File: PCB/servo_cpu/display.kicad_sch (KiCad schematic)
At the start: 15 parts, among them SW1 ENTER, SW2 ESC, SW3 UP, SW4 DOWN

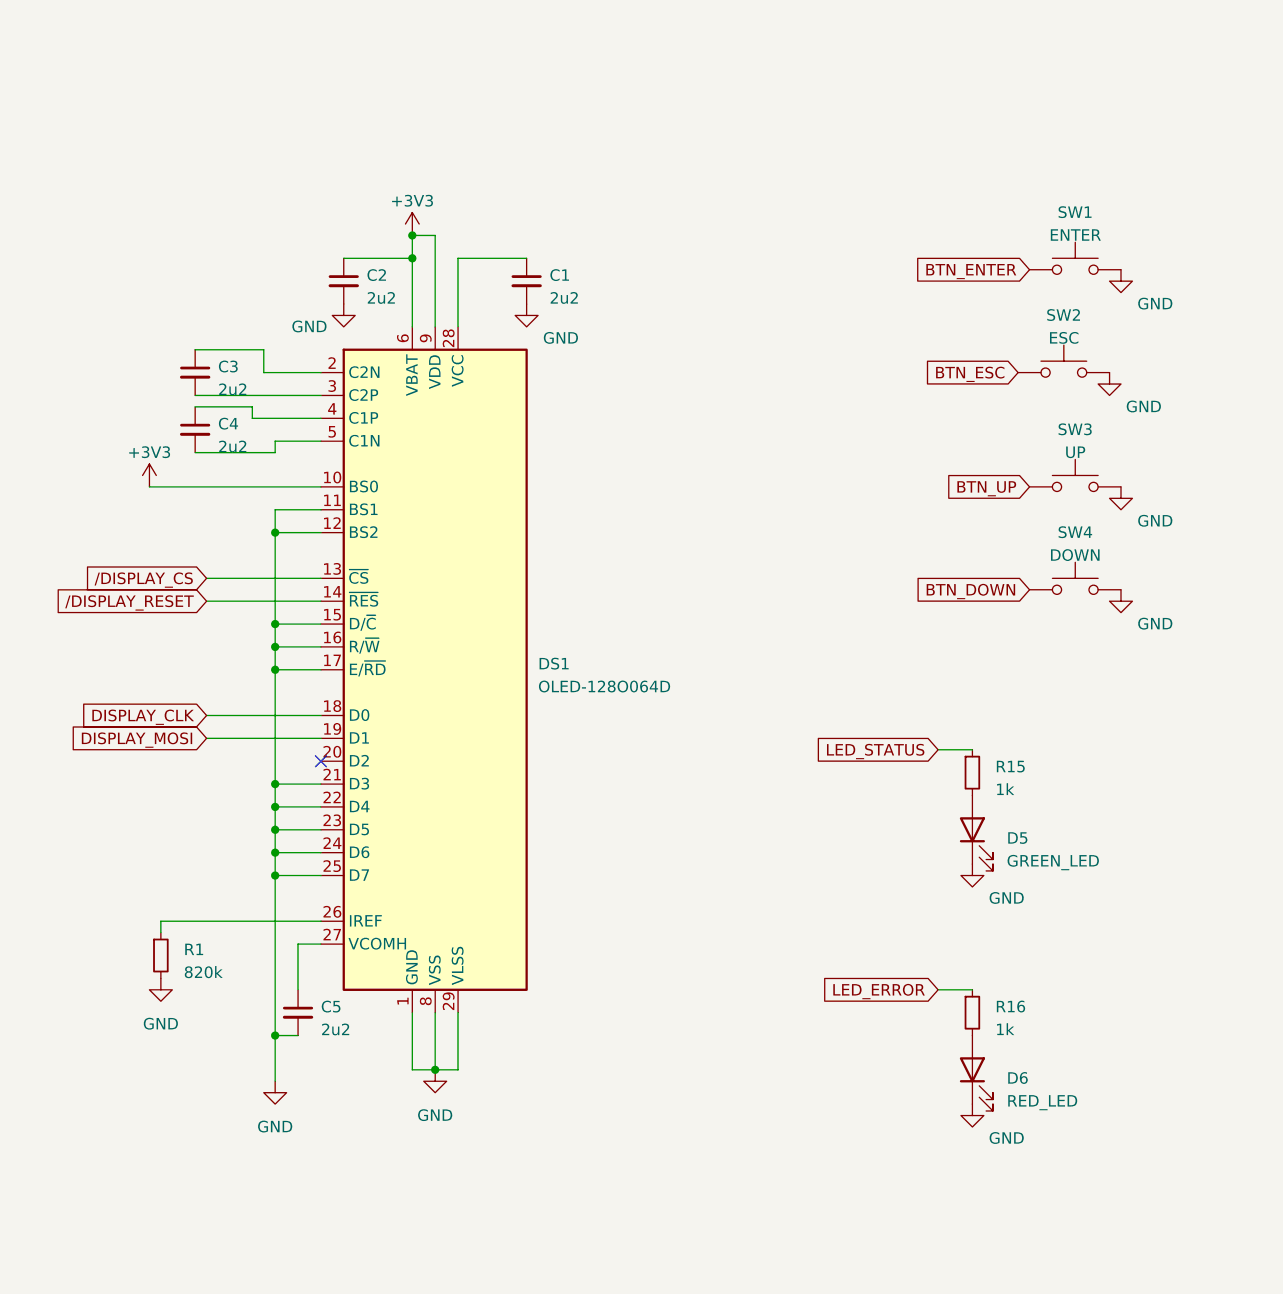
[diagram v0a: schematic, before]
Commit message: CPU schematic done
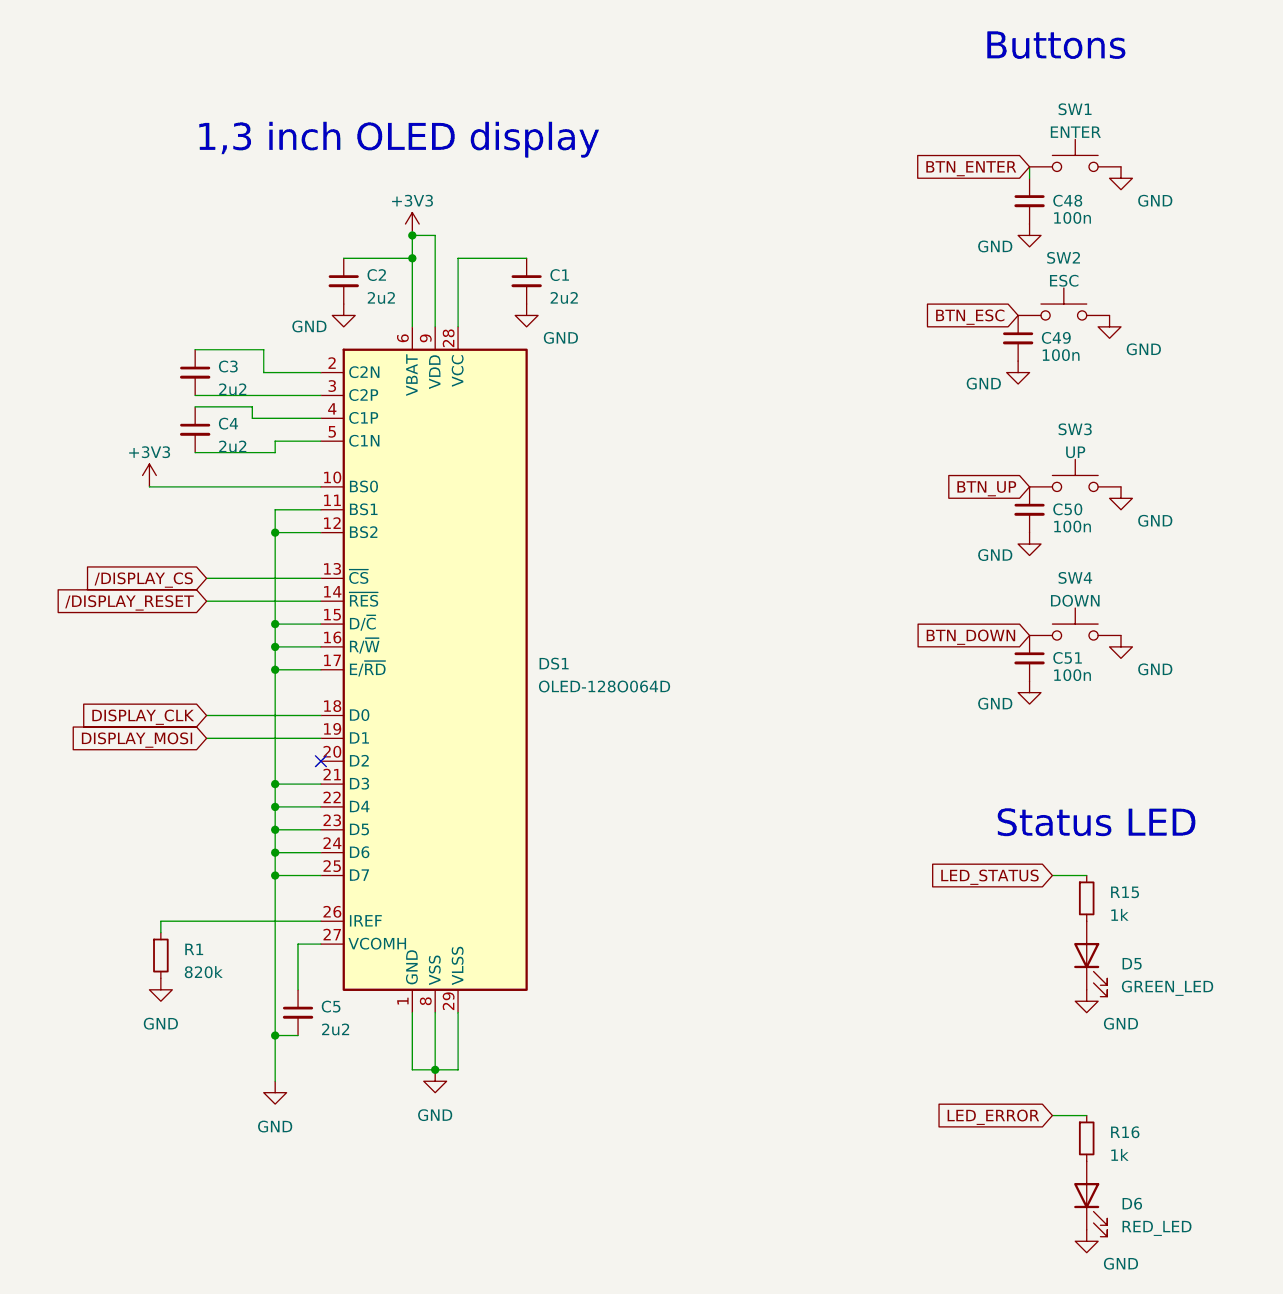
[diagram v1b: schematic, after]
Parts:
- added C48, C49, C50, C51: 100n, symbol Device:C_Small
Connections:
- net BTN_DOWN: now also C51.1
- net BTN_ENTER: now also C48.1
- net BTN_ESC: now also C49.1
- net BTN_UP: now also C50.1
- net GND: now also C48.2, C49.2, C50.2, C51.2
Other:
- note added: "1,3 inch OLED display"
- note added: "Buttons"
- note added: "Status LED"
- title: (none) -> Display
- moved on the sheet: D5, D6, R15, R16, SW1, SW2, SW4

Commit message: cpu pcb layout
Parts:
- C1, C2, C3, C4, C48, C49, C5, C50, C51: footprint (none) -> Capacitor_SMD:C_0805_2012Metric_Pad1.18x1.45mm_HandSolder
- R1, R15, R16: footprint (none) -> Resistor_SMD:R_0805_2012Metric_Pad1.20x1.40mm_HandSolder
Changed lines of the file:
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@@
       (effects (font (size 1.27 1.27)) (justify left))
     )
-    (property "Footprint" "" (at 134.62 86.36 0)
+    (property "Footprint" "Capacitor_SMD:C_0805_2012Metric_Pad1.18x1.45mm_HandSolder" (at 134.62 86.36 0)
       (effects (font (size 1.27 1.27)) hide)
     )
@@
       (effects (font (size 1.27 1.27)) (justify left))
     )
-    (property "Footprint" "" (at 134.62 35.56 0)
+    (property "Footprint" "Capacitor_SMD:C_0805_2012Metric_Pad1.18x1.45mm_HandSolder" (at 134.62 35.56 0)
       (effects (font (size 1.27 1.27)) hide)
     )
@@
       (effects (font (size 1.27 1.27)) (justify left))
     )
-    (property "Footprint" "" (at 41.91 60.96 0)
+    (property "Footprint" "Capacitor_SMD:C_0805_2012Metric_Pad1.18x1.45mm_HandSolder" (at 41.91 60.96 0)
       (effects (font (size 1.27 1.27)) hide)
     )
@@
       (effects (font (size 1.27 1.27)) (justify left))
     )
-    (property "Footprint" "" (at 134.62 69.85 0)
+    (property "Footprint" "Capacitor_SMD:C_0805_2012Metric_Pad1.18x1.45mm_HandSolder" (at 134.62 69.85 0)
       (effects (font (size 1.27 1.27)) hide)
     )
@@
       (effects (font (size 1.27 1.27)) (justify left))
     )
-    (property "Footprint" "" (at 78.74 44.45 0)
+    (property "Footprint" "Capacitor_SMD:C_0805_2012Metric_Pad1.18x1.45mm_HandSolder" (at 78.74 44.45 0)
       (effects (font (size 1.27 1.27)) hide)
     )
@@
       (effects (font (size 1.27 1.27)) (justify left))
     )
-    (property "Footprint" "" (at 53.34 125.73 0)
+    (property "Footprint" "Capacitor_SMD:C_0805_2012Metric_Pad1.18x1.45mm_HandSolder" (at 53.34 125.73 0)
       (effects (font (size 1.27 1.27)) hide)
     )
@@
       (effects (font (size 1.27 1.27)) (justify left))
     )
-    (property "Footprint" "" (at 140.97 113.03 0)
+    (property "Footprint" "Resistor_SMD:R_0805_2012Metric_Pad1.20x1.40mm_HandSolder" (at 140.97 113.03 0)
       (effects (font (size 1.27 1.27)) hide)
     )
@@
       (effects (font (size 1.27 1.27)) (justify left))
     )
-    (property "Footprint" "" (at 133.35 50.8 0)
+    (property "Footprint" "Capacitor_SMD:C_0805_2012Metric_Pad1.18x1.45mm_HandSolder" (at 133.35 50.8 0)
       (effects (font (size 1.27 1.27)) hide)
     )
@@
       (effects (font (size 1.27 1.27)) (justify left))
     )
-    (property "Footprint" "" (at 140.97 139.7 0)
+    (property "Footprint" "Resistor_SMD:R_0805_2012Metric_Pad1.20x1.40mm_HandSolder" (at 140.97 139.7 0)
       (effects (font (size 1.27 1.27)) hide)
     )
@@
       (effects (font (size 1.27 1.27)) (justify left))
     )
-    (property "Footprint" "" (at 38.1 119.38 0)
+    (property "Footprint" "Resistor_SMD:R_0805_2012Metric_Pad1.20x1.40mm_HandSolder" (at 38.1 119.38 0)
       (effects (font (size 1.27 1.27)) hide)
     )
@@
       (effects (font (size 1.27 1.27)) (justify left))
     )
-    (property "Footprint" "" (at 41.91 54.61 0)
+    (property "Footprint" "Capacitor_SMD:C_0805_2012Metric_Pad1.18x1.45mm_HandSolder" (at 41.91 54.61 0)
       (effects (font (size 1.27 1.27)) hide)
     )
@@
       (effects (font (size 1.27 1.27)) (justify left))
     )
-    (property "Footprint" "" (at 58.42 44.45 0)
-      (effects (font (size 1.27 1.27)) hide)
-    )
+    (property "Footprint" "Capacitor_SMD:C_0805_2012Metric_Pad1.18x1.45mm_HandSolder" (at 58.42 44.45 0)
+      (effects (font (size 1.27 1.27)) hide)
+    )
